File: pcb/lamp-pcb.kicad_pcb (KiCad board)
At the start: 2 copper layers, 105.4 x 91.4 mm, 41 parts, among them IC1 ATMEGA328P, IC2 LM1117, IC3 TLC5973, J1 5V_OUT, J2 LED_CARD_BOTTOM, M2 Val**, P1 7-12V_IN, P2 AVR_ISP, P3 SERIAL, P4 LEDSTACK, P5 LEDSTACK, P6 LEDSTACK, P7 LED_CARD_TOP, P8 SER_SHORT, Y1 14.7456MHz

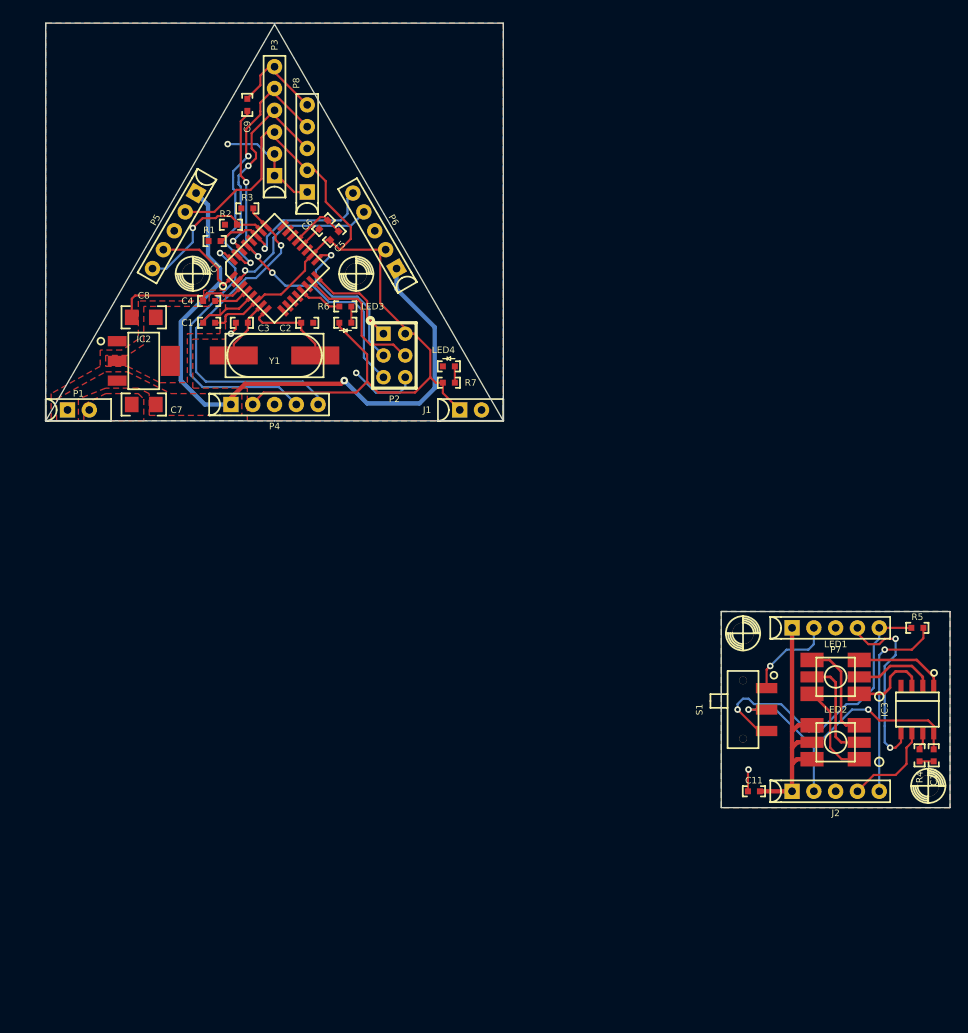
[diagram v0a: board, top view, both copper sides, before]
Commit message: got some panelization going on for quotes
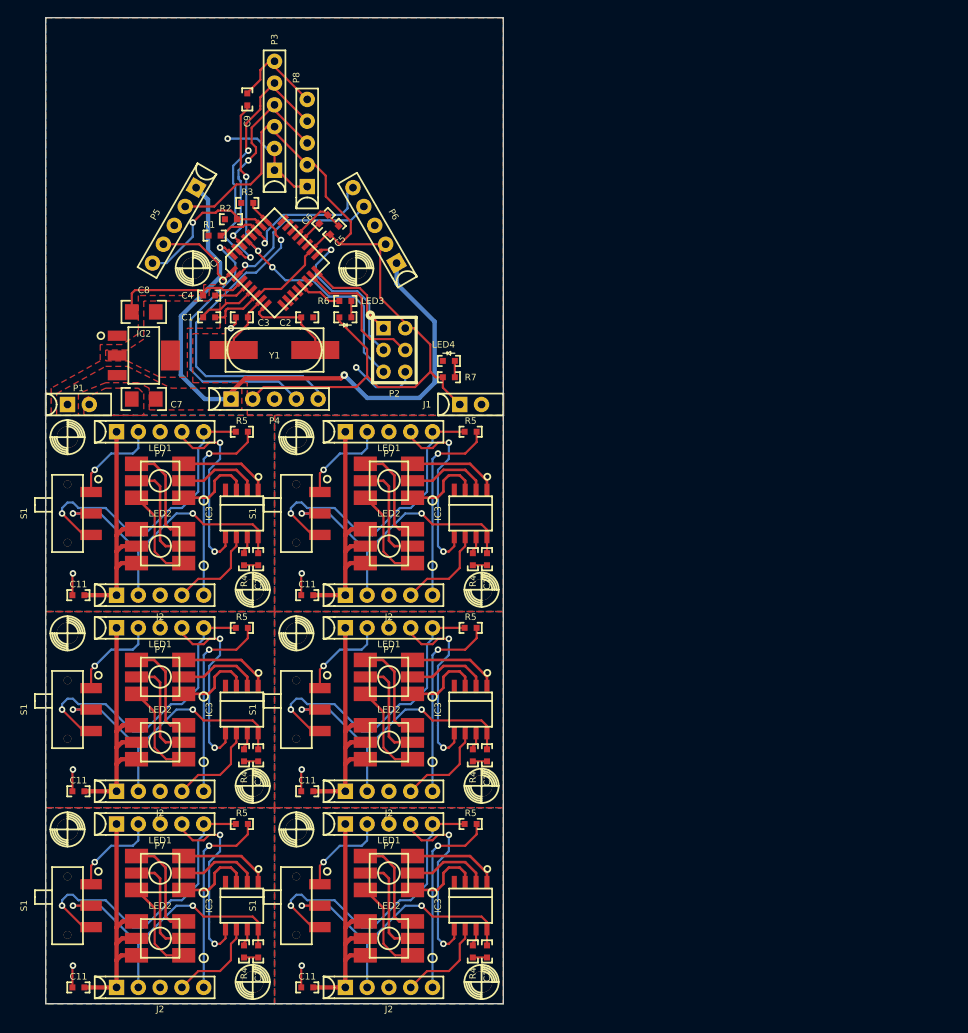
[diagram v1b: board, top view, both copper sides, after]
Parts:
- added C10: 0.1uF, passive-smd:0603(1608m), F.Cu at (98.4, 141.2)
- added C10: 0.1uF, passive-smd:0603(1608m), F.Cu at (125.1, 141.2)
- added C10: 0.1uF, passive-smd:0603(1608m), F.Cu at (98.4, 164.1)
- added C10: 0.1uF, passive-smd:0603(1608m), F.Cu at (125.1, 164.1)
- added C10: 0.1uF, passive-smd:0603(1608m), F.Cu at (125.1, 118.4)
- added C11: 0.1uF, passive-smd:0603(1608m), F.Cu at (77.5, 145.4)
- added C11: 0.1uF, passive-smd:0603(1608m), F.Cu at (104.1, 145.4)
- added C11: 0.1uF, passive-smd:0603(1608m), F.Cu at (77.5, 168.3)
- added C11: 0.1uF, passive-smd:0603(1608m), F.Cu at (104.1, 168.3)
- added C11: 0.1uF, passive-smd:0603(1608m), F.Cu at (104.1, 122.6)
- added IC3: TLC5973, soic:SOIC8, F.Cu at (96.5, 135.9)
- added IC3: TLC5973, soic:SOIC8, F.Cu at (123.2, 135.9)
- added IC3: TLC5973, soic:SOIC8, F.Cu at (96.5, 158.8)
- added IC3: TLC5973, soic:SOIC8, F.Cu at (123.2, 158.8)
- added IC3: TLC5973, soic:SOIC8, F.Cu at (123.2, 113.0)
- added J2: LED_CARD_BOTTOM, sip:SIP5, F.Cu at (87.0, 145.4)
- added J2: LED_CARD_BOTTOM, sip:SIP5, F.Cu at (113.7, 145.4)
- added J2: LED_CARD_BOTTOM, sip:SIP5, F.Cu at (87.0, 168.3)
- added J2: LED_CARD_BOTTOM, sip:SIP5, F.Cu at (113.7, 168.3)
- added J2: LED_CARD_BOTTOM, sip:SIP5, F.Cu at (113.7, 122.6)
- added LED1: CREE-CLV6A-FKB, led:PLCC6-SM-RGB-LED, F.Cu at (87.0, 132.1)
- added LED1: CREE-CLV6A-FKB, led:PLCC6-SM-RGB-LED, F.Cu at (113.7, 132.1)
- added LED1: CREE-CLV6A-FKB, led:PLCC6-SM-RGB-LED, F.Cu at (87.0, 154.9)
- added LED1: CREE-CLV6A-FKB, led:PLCC6-SM-RGB-LED, F.Cu at (113.7, 154.9)
- added LED1: CREE-CLV6A-FKB, led:PLCC6-SM-RGB-LED, F.Cu at (113.7, 109.2)
- added LED2: CREE-CLV6A-FKB, led:PLCC6-SM-RGB-LED, F.Cu at (87.0, 139.7)
- added LED2: CREE-CLV6A-FKB, led:PLCC6-SM-RGB-LED, F.Cu at (113.7, 139.7)
- added LED2: CREE-CLV6A-FKB, led:PLCC6-SM-RGB-LED, F.Cu at (87.0, 162.6)
- added LED2: CREE-CLV6A-FKB, led:PLCC6-SM-RGB-LED, F.Cu at (113.7, 162.6)
- added LED2: CREE-CLV6A-FKB, led:PLCC6-SM-RGB-LED, F.Cu at (113.7, 116.8)
- added M2: Val**, asm:M2, F.Cu at (76.2, 127.0)
- added M2: Val**, asm:M2, F.Cu at (124.5, 121.9)
- added M2: Val**, asm:M2, F.Cu at (97.8, 144.8)
- added M2: Val**, asm:M2, F.Cu at (124.5, 144.8)
- added M2: Val**, asm:M2, F.Cu at (102.9, 127.0)
- added M2: Val**, asm:M2, F.Cu at (76.2, 149.9)
- added M2: Val**, asm:M2, F.Cu at (97.8, 167.6)
- added M2: Val**, asm:M2, F.Cu at (124.5, 167.6)
- added M2: Val**, asm:M2, F.Cu at (102.9, 149.9)
- added M2: Val**, asm:M2, F.Cu at (102.9, 104.1)
- added P7: LED_CARD_TOP, sip:SIP5, F.Cu at (87.0, 126.4)
- added P7: LED_CARD_TOP, sip:SIP5, F.Cu at (113.7, 126.4)
- added P7: LED_CARD_TOP, sip:SIP5, F.Cu at (87.0, 149.2)
- added P7: LED_CARD_TOP, sip:SIP5, F.Cu at (113.7, 149.2)
- added P7: LED_CARD_TOP, sip:SIP5, F.Cu at (113.7, 103.5)
- added R4: 2kΩ, passive-smd:0603(1608m), F.Cu at (96.8, 141.2)
- added R4: 2kΩ, passive-smd:0603(1608m), F.Cu at (123.4, 141.2)
- added R4: 2kΩ, passive-smd:0603(1608m), F.Cu at (96.8, 164.1)
- added R4: 2kΩ, passive-smd:0603(1608m), F.Cu at (123.4, 164.1)
- added R4: 2kΩ, passive-smd:0603(1608m), F.Cu at (123.4, 118.4)
- added R5: 1kΩ, passive-smd:0603(1608m), F.Cu at (96.5, 126.4)
- added R5: 1kΩ, passive-smd:0603(1608m), F.Cu at (123.2, 126.4)
- added R5: 1kΩ, passive-smd:0603(1608m), F.Cu at (96.5, 149.2)
- added R5: 1kΩ, passive-smd:0603(1608m), F.Cu at (123.2, 149.2)
- added R5: 1kΩ, passive-smd:0603(1608m), F.Cu at (123.2, 103.5)
- added S1: TOP, switch:CK-JS102011SAQN_sm-spdt-switch, F.Cu at (76.2, 135.9)
- added S1: TOP, switch:CK-JS102011SAQN_sm-spdt-switch, F.Cu at (102.9, 135.9)
- added S1: TOP, switch:CK-JS102011SAQN_sm-spdt-switch, F.Cu at (76.2, 158.8)
- added S1: TOP, switch:CK-JS102011SAQN_sm-spdt-switch, F.Cu at (102.9, 158.8)
- added S1: TOP, switch:CK-JS102011SAQN_sm-spdt-switch, F.Cu at (102.9, 113.0)
- moved LED1 82.0 mm to (87.0, 109.2)
- moved P7 82.0 mm to (87.0, 103.5)
- moved M2 82.0 mm to (97.8, 121.9)
- moved M2 82.0 mm to (76.2, 104.1)
- moved R5 82.0 mm to (96.5, 103.5)
- moved C11 82.0 mm to (77.5, 122.6)
- moved J2 82.0 mm to (87.0, 122.6)
- moved LED2 82.0 mm to (87.0, 116.8)
- moved R4 82.0 mm to (96.8, 118.4)
- moved C10 82.0 mm to (98.4, 118.4)
- moved IC3 82.0 mm to (96.5, 113.0)
- moved S1 82.0 mm to (76.2, 113.0)
- moved C1 0.64 mm to (92.7, 90.2)
- moved C2 0.64 mm to (104.1, 90.2)
- moved C3 0.64 mm to (96.5, 90.2)
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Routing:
- net /VLOG: track 36.0 -> 215.9 mm, vias 2 -> 12
- net /SENSE_TOP: track 35.9 -> 215.2 mm, vias 1 -> 6
- net /VLED: track 30.6 -> 183.4 mm
- net /SENSE_BOT: track 23.0 -> 138.2 mm, vias 1 -> 6
- net /LED_SER_OUT: track 22.0 -> 132.0 mm, vias 2 -> 12
- net Net-(LED1-Pad5): track 12.4 -> 74.3 mm
- net Net-(LED1-Pad4): track 12.0 -> 72.0 mm
- net Net-(LED1-Pad6): track 11.1 -> 66.6 mm
- net /LED_SER_IN: track 10.9 -> 65.7 mm
- net /VLOG_TOP: track 10.8 -> 64.8 mm, vias 1 -> 6
- net /RED: track 10.6 -> 63.6 mm
- net /GRN: track 9.57 -> 57.4 mm
- net /BLU: track 9.34 -> 56.0 mm
- net /LED_GND: track 4.22 -> 25.3 mm, vias 1 -> 6
- net Net-(IC3-Pad7): track 2.09 -> 12.6 mm
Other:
- board size 105.4 x 91.4 mm -> 53.3 x 114.9 mm
